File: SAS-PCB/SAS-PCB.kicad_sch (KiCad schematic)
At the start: 8 parts, among them J1 Conn_SMA_RF2-04A-T-00-50-G, J1-BMP280 Conn_01x06_Pin, J2 Conn_02x20_Odd_Even, J3-GPS Conn_01x04_Socket, J4-LCD1 Conn_01x04_Socket, J5-LCD2 Conn_01x04_Socket, J6-FAN1 Conn_01x02_Pin, J7-FAN2 Conn_01x02_Pin

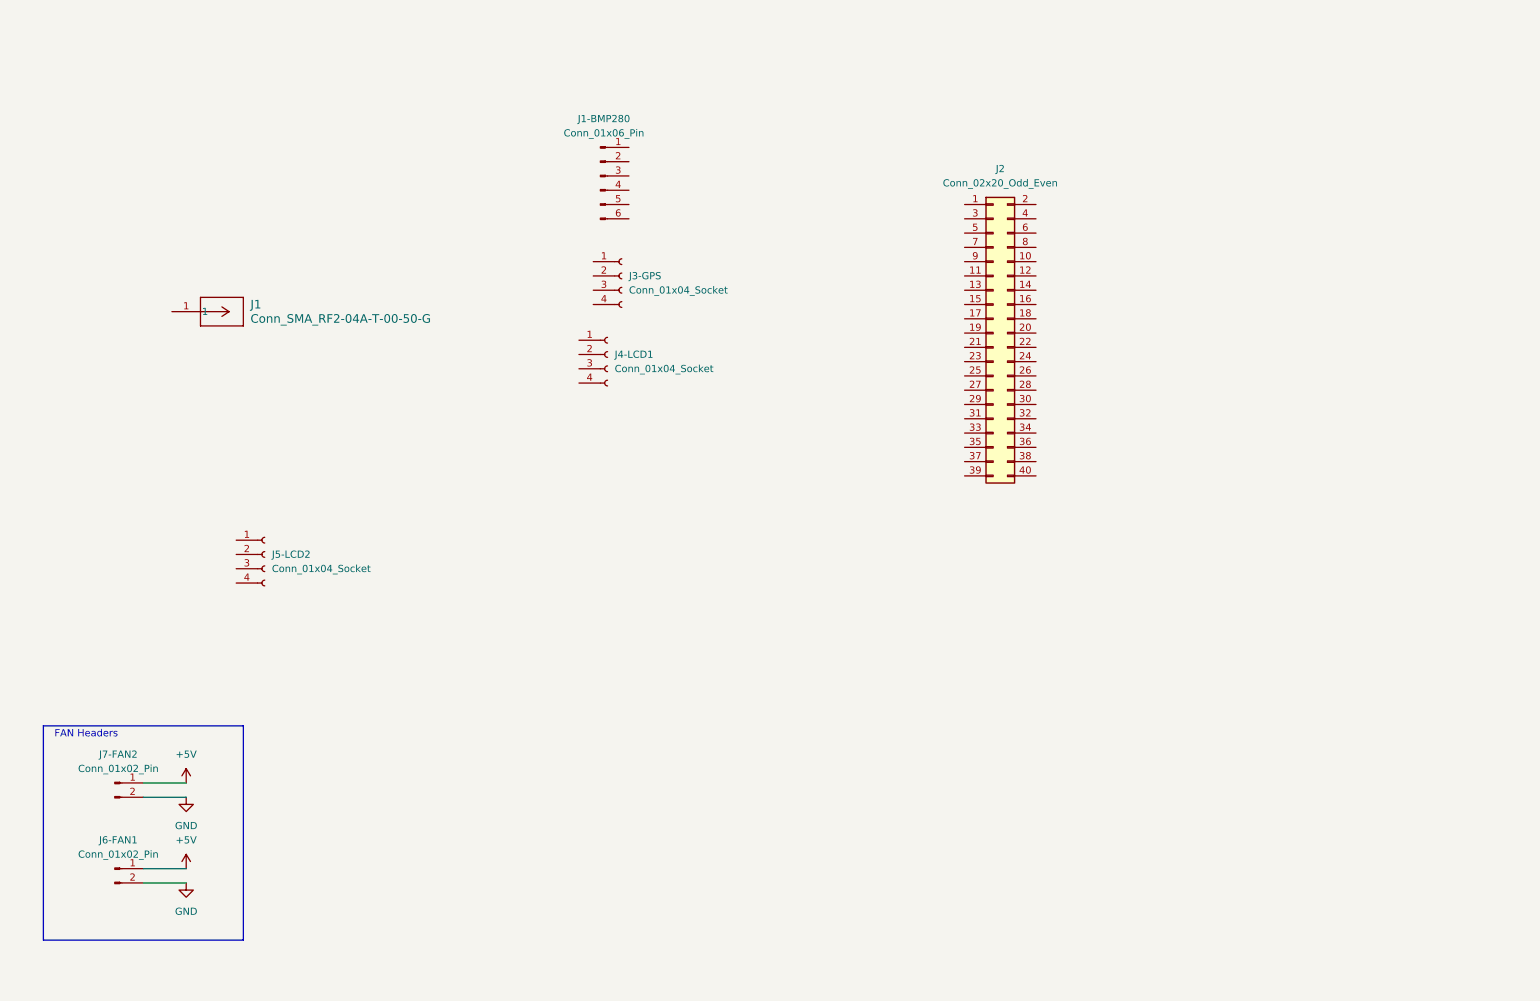
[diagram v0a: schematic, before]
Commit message: schematic done
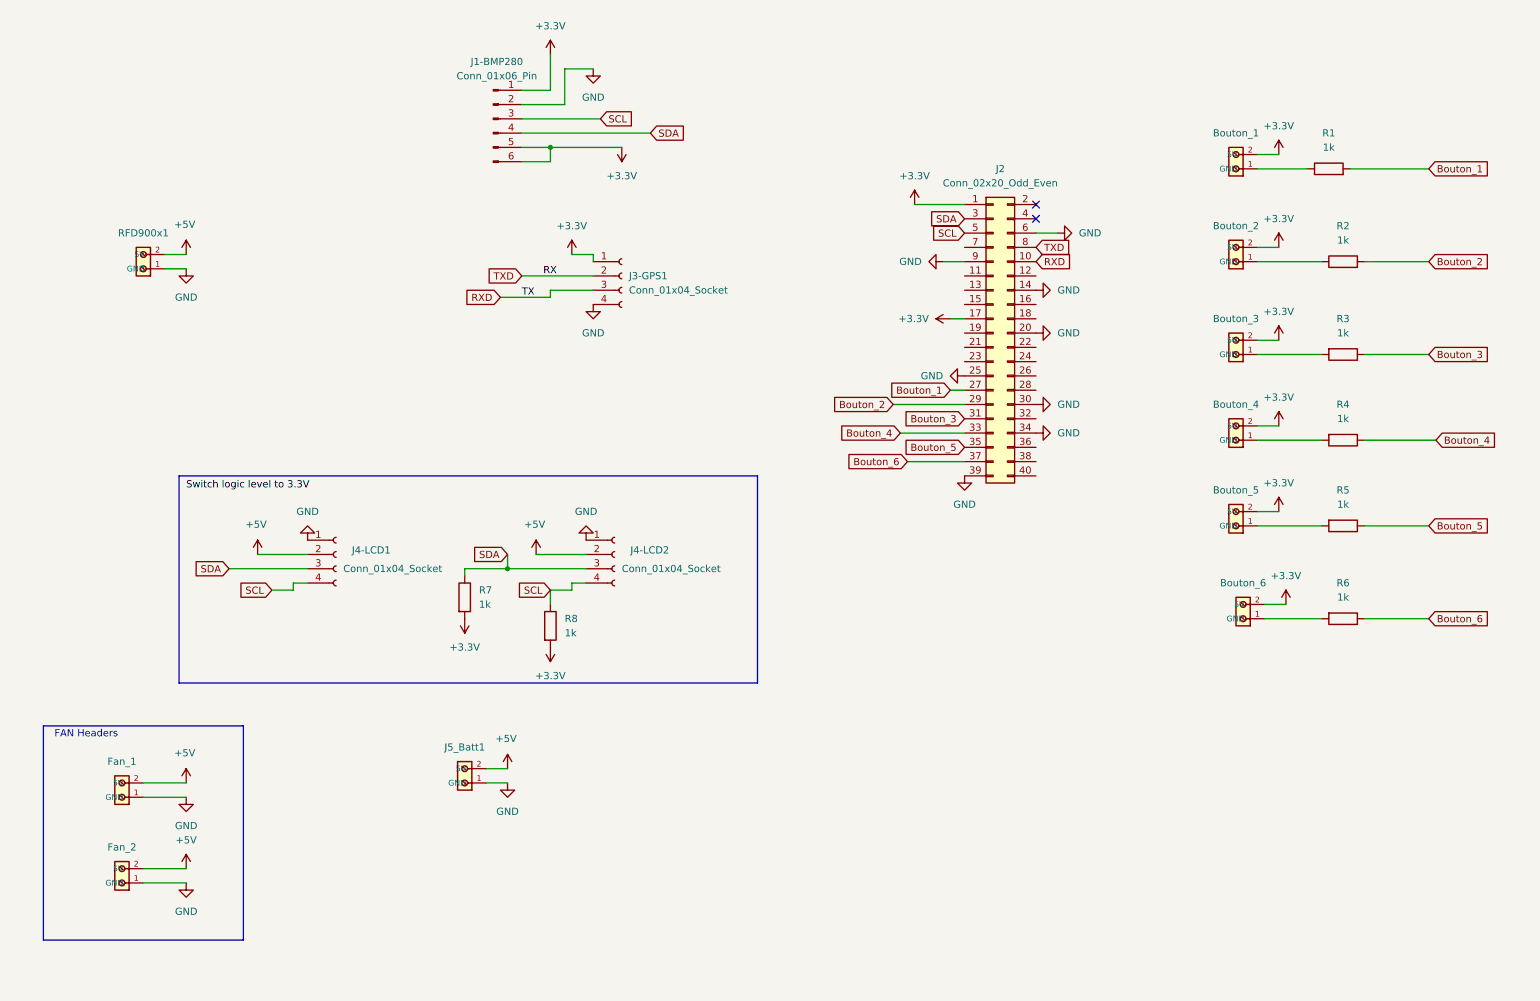
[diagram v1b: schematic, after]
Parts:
- removed J1: Conn_SMA_RF2-04A-T-00-50-G, CONN_RF2-04A-T-00-50-G_ADM, symbol SAS-librairie_symboles:Conn_SMA_RF2-04A-T-00-50-G
- removed J5-LCD2: Conn_01x04_Socket, symbol Connector:Conn_01x04_Socket
- removed J6-FAN1, J7-FAN2: Conn_01x02_Pin, symbol Connector:Conn_01x02_Pin
- added Bouton_1, Bouton_2, Bouton_3, Bouton_4, Bouton_5, Bouton_6, Fan_1, Fan_2, J5_Batt1, RFD900x1: 691137710002, SAS-Librarie-Empreinte:bornie_2position, symbol SAS-librairie_symboles:bornier_2position
- added J4-LCD2: Conn_01x04_Socket, SAS-Librarie-Empreinte:Conn_4_pos, symbol Connector:Conn_01x04_Socket
- added R1, R2, R3, R4, R5, R6, R7, R8: 1k, SAS-Librarie-Empreinte:Resistance, symbol Device:R
- J1-BMP280: footprint (none) -> SAS-Librarie-Empreinte:Conn_6_pos
- J2: footprint (none) -> Connector_PinSocket_2.54mm:PinSocket_2x20_P2.54mm_Vertical
- J3-GPS1: renamed from J3-GPS; footprint (none) -> SAS-Librarie-Empreinte:Conn_4_pos
- J4-LCD1: footprint (none) -> SAS-Librarie-Empreinte:Conn_4_pos
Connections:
- net +5V: now also J4-LCD1.2 (Pin_2), Fan_1.2 (5V), Fan_2.2 (5V), J4-LCD2.2 (Pin_2), J5_Batt1.2 (5V), RFD900x1.2 (5V)
- net GND: now also J1-BMP280.2 (Pin_2), J2.14 (Pin_14), J2.20 (Pin_20), J2.25 (Pin_25), J2.30 (Pin_30), J2.34 (Pin_34), J2.39 (Pin_39), J2.6 (Pin_6), J2.9 (Pin_9), J3-GPS1.4 (Pin_4), J4-LCD1.1 (Pin_1), Fan_1.1 (GND), Fan_2.1 (GND), J4-LCD2.1 (Pin_1), J5_Batt1.1 (GND), RFD900x1.1 (GND)
- net +3.3V: now reaches J3-GPS1.1 (Pin_1)
- net +3.3V: now also J1-BMP280.1 (Pin_1), J1-BMP280.5 (Pin_5), J1-BMP280.6 (Pin_6), J2.1 (Pin_1), J2.17 (Pin_17), Bouton_1.2 (5V), Bouton_2.2 (5V), Bouton_3.2 (5V), Bouton_4.2 (5V), Bouton_5.2 (5V), Bouton_6.2 (5V), R7.2, R8.2
- net TXD: now reaches J3-GPS1.2 (Pin_2)
- net TXD: now also J2.8 (Pin_8)
- net RXD: now reaches J3-GPS1.3 (Pin_3)
- net RXD: now also J2.10 (Pin_10)
- net Bouton_1: now reaches J2.27 (Pin_27)
- net Bouton_1: now also R1.2
- net Bouton_2: now reaches J2.29 (Pin_29)
- net Bouton_2: now also R2.2
- net SDA: now reaches J2.3 (Pin_3)
- net SDA: now also J1-BMP280.4 (Pin_4), J4-LCD1.3 (Pin_3), J4-LCD2.3 (Pin_3), R7.1
- net Bouton_3: now reaches J2.31 (Pin_31)
- net Bouton_3: now also R3.1
- net Bouton_4: now reaches J2.33 (Pin_33)
- net Bouton_4: now also R4.1
- net Bouton_5: now reaches J2.35 (Pin_35)
- net Bouton_5: now also R5.1
- net Bouton_6: now reaches J2.37 (Pin_37)
- net Bouton_6: now also R6.1
- net SCL: now reaches J2.5 (Pin_5)
- net SCL: now also J1-BMP280.3 (Pin_3), J4-LCD1.4 (Pin_4), J4-LCD2.4 (Pin_4), R8.1
- new net: Bouton_6.1 (GND), R6.2
- new net: Bouton_5.1 (GND), R5.2
- new net: Bouton_2.1 (GND), R2.1
- new net: Bouton_1.1 (GND), R1.1
- new net: Bouton_4.1 (GND), R4.2
- new net: Bouton_3.1 (GND), R3.2
- no-connect marks 0 -> 2
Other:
- moved on the sheet: J1-BMP280, J4-LCD1

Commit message: Rooting terminé
Reste à refaire les mounting holes et enlever les bouttes de cuivre trop mince.
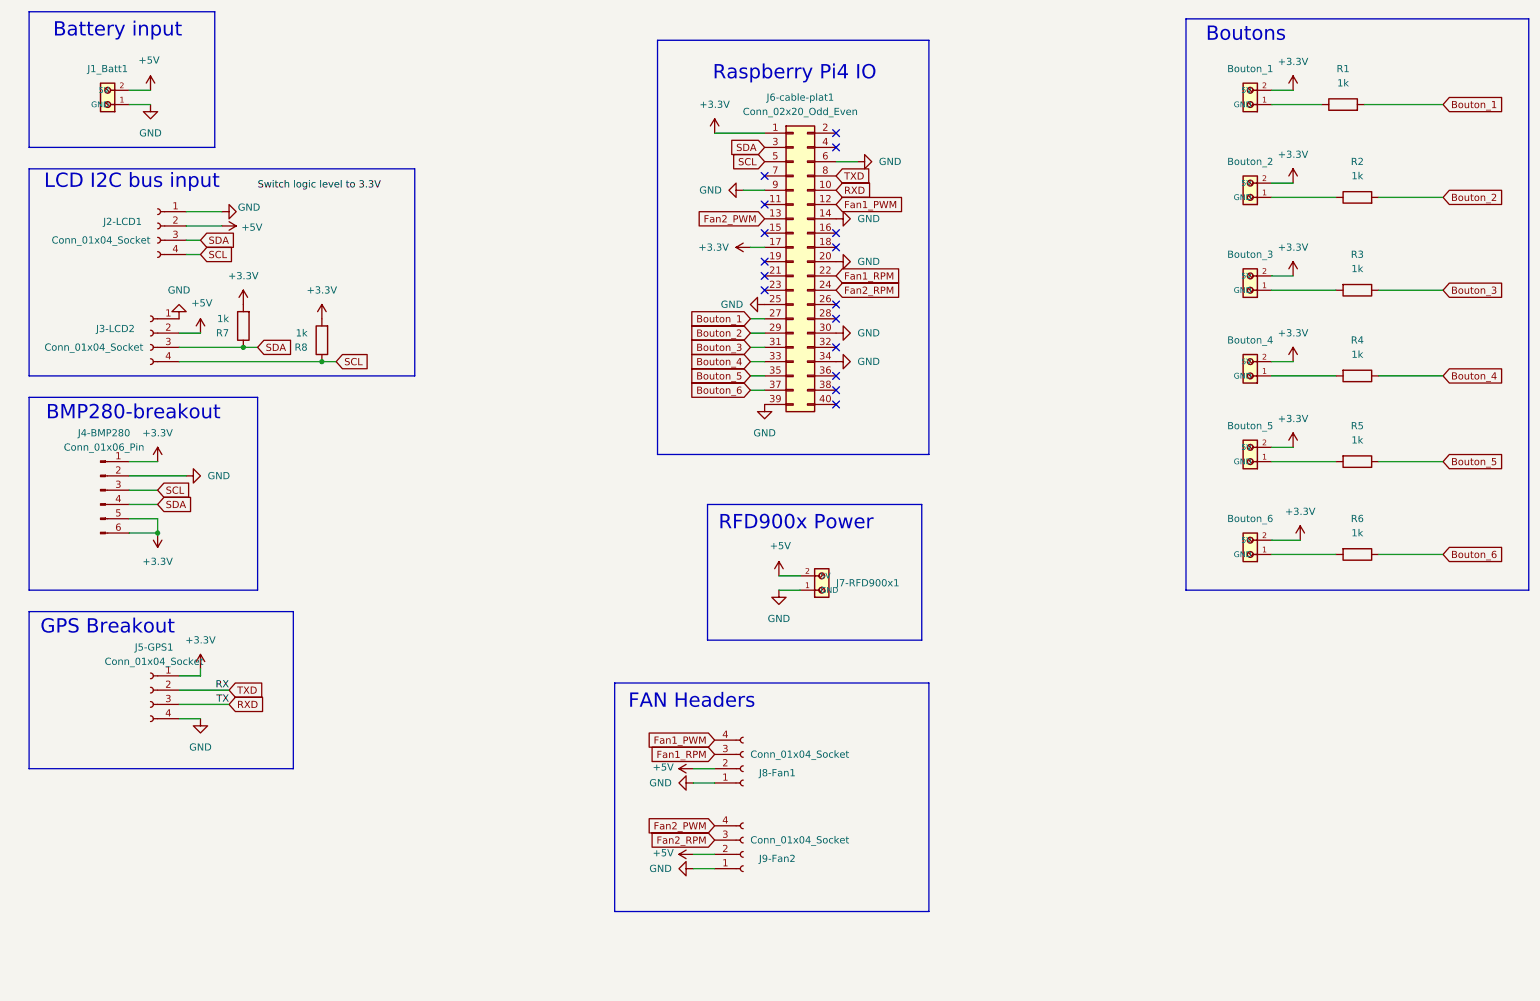
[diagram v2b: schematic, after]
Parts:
- removed Fan_1, Fan_2: 691137710002, SAS-Librarie-Empreinte:bornie_2position, symbol SAS-librairie_symboles:bornier_2position
- added J8-Fan1, J9-Fan2: Conn_01x04_Socket, SAS-Librarie-Empreinte:Conn_4_pos, symbol Connector:Conn_01x04_Socket
- J4-BMP280: renamed from J1-BMP280; footprint SAS-Librarie-Empreinte:Conn_6_pos -> SAS-Librarie-Empreinte:Header-BMP280
- J5-GPS1: renamed from J3-GPS1; footprint SAS-Librarie-Empreinte:Conn_4_pos -> SAS-Librarie-Empreinte:conn-GPS
- renumbered J5_Batt1 to J1_Batt1, J4-LCD1 to J2-LCD1, J4-LCD2 to J3-LCD2, J2 to J6-cable-plat1, RFD900x1 to J7-RFD900x1
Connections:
- net +5V: now also J8-Fan1.2 (Pin_2), J9-Fan2.2 (Pin_2)
- net GND: now also J8-Fan1.1 (Pin_1), J9-Fan2.1 (Pin_1)
- net Fan1_PWM: now reaches J6-cable-plat1.12 (Pin_12)
- net Fan1_PWM: now also J8-Fan1.4 (Pin_4)
- net Fan2_PWM: now reaches J6-cable-plat1.13 (Pin_13)
- net Fan2_PWM: now also J9-Fan2.4 (Pin_4)
- net Fan1_RPM: now reaches J6-cable-plat1.22 (Pin_22)
- net Fan1_RPM: now also J8-Fan1.3 (Pin_3)
- net Fan2_RPM: now reaches J6-cable-plat1.24 (Pin_24)
- net Fan2_RPM: now also J9-Fan2.3 (Pin_3)
- no-connect marks 2 -> 16
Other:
- note added: "BMP280-breakout"
- note added: "Battery input"
- note added: "Boutons"
- note added: "GPS Breakout"
- note added: "LCD I2C bus input"
- note added: "RFD900x Power"
- note added: "Raspberry Pi4 IO"
- moved on the sheet: Bouton_1, Bouton_2, Bouton_3, Bouton_4, Bouton_5, Bouton_6, J1_Batt1, J2-LCD1, J3-LCD2, J4-BMP280, J5-GPS1, J6-cable-plat1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

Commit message: Header Fix
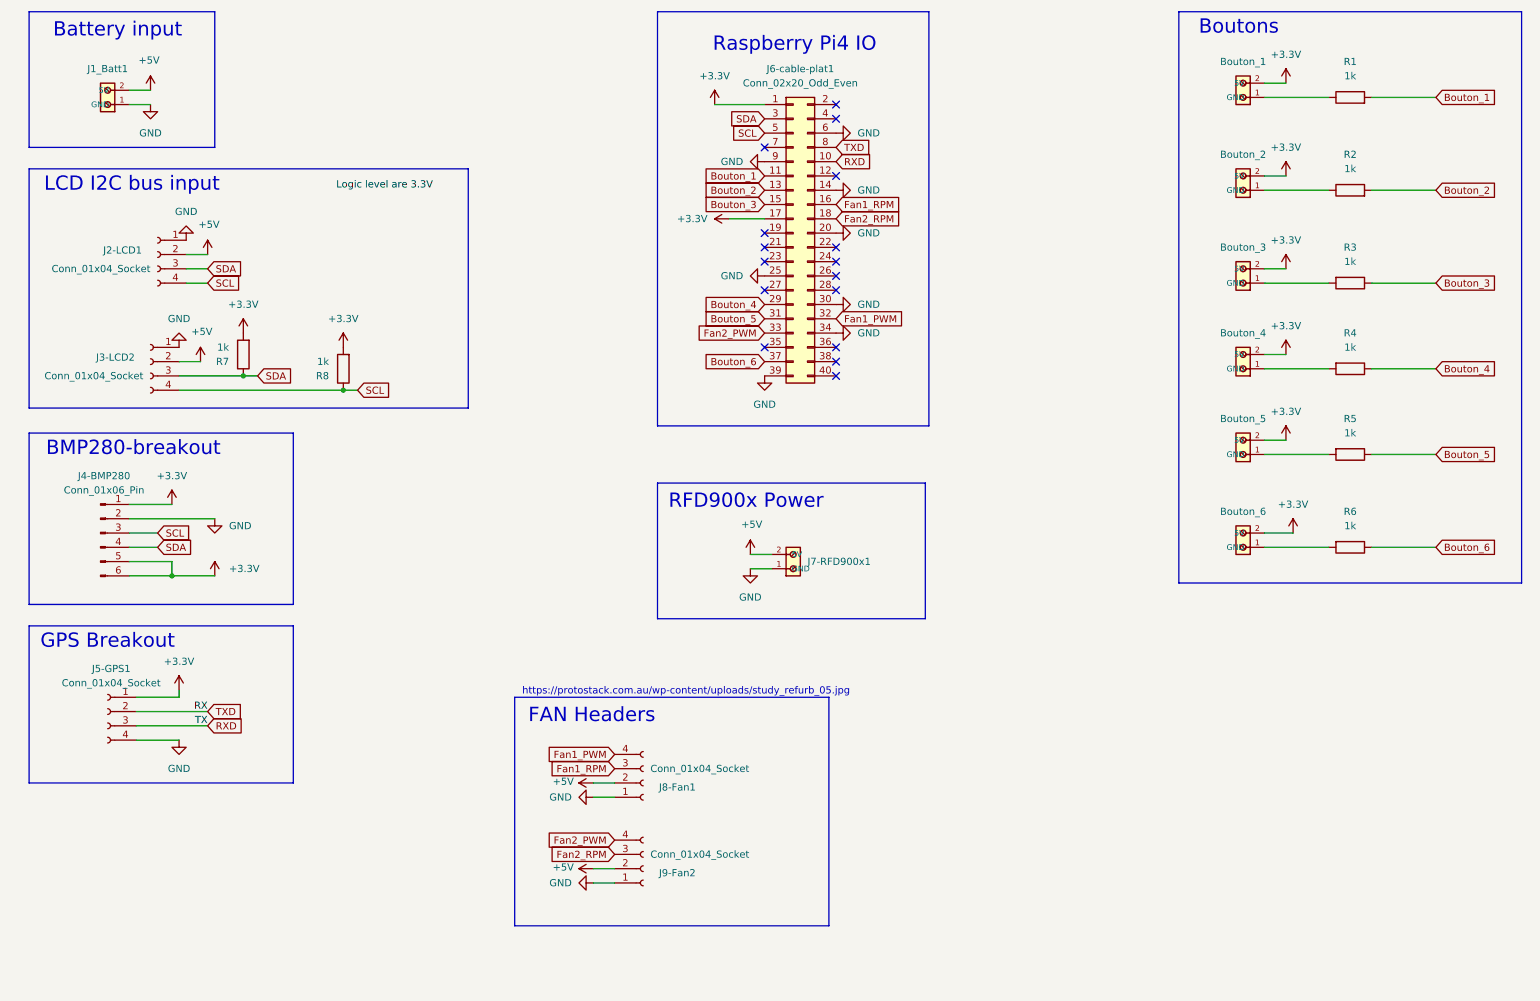
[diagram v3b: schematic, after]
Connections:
- net Bouton_1: now also J6-cable-plat1.11 (Pin_11); no longer J6-cable-plat1.27 (Pin_27)
- net Bouton_2: now also J6-cable-plat1.13 (Pin_13); no longer J6-cable-plat1.29 (Pin_29)
- net Bouton_3: now also J6-cable-plat1.15 (Pin_15); no longer J6-cable-plat1.31 (Pin_31)
- net Bouton_4: now also J6-cable-plat1.29 (Pin_29); no longer J6-cable-plat1.33 (Pin_33)
- net Bouton_5: now also J6-cable-plat1.31 (Pin_31); no longer J6-cable-plat1.35 (Pin_35)
- net Fan1_PWM: now also J6-cable-plat1.32 (Pin_32); no longer J6-cable-plat1.12 (Pin_12)
- net Fan1_RPM: now also J6-cable-plat1.16 (Pin_16); no longer J6-cable-plat1.22 (Pin_22)
- net Fan2_PWM: now also J6-cable-plat1.33 (Pin_33); no longer J6-cable-plat1.13 (Pin_13)
- net Fan2_RPM: now also J6-cable-plat1.18 (Pin_18); no longer J6-cable-plat1.24 (Pin_24)
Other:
- note added: "https://protostack.com.au/wp-content/uploads/study_refurb_05.jpg"
- moved on the sheet: Bouton_1, Bouton_2, Bouton_3, Bouton_4, Bouton_5, Bouton_6, J2-LCD1, J3-LCD2, J4-BMP280, J5-GPS1, J6-cable-plat1, J7-RFD900x1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

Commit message: u1
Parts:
- J1_Batt1, J7-RFD900x1: footprint SAS-Librarie-Empreinte:bornie_2position -> SAS-Librarie-Empreinte:AMASS_XT30U-F_1x02_P5.0mm_Vertical
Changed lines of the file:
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@@
 			)
 		)
-		(property "Footprint" "SAS-Librarie-Empreinte:bornie_2position"
+		(property "Footprint" "SAS-Librarie-Empreinte:AMASS_XT30U-F_1x02_P5.0mm_Vertical"
 			(at 152.4 111.76 0)
 			(effects
@@
 			)
 		)
-		(property "Footprint" "SAS-Librarie-Empreinte:bornie_2position"
+		(property "Footprint" "SAS-Librarie-Empreinte:AMASS_XT30U-F_1x02_P5.0mm_Vertical"
 			(at 27.94 29.21 0)
 			(effects
